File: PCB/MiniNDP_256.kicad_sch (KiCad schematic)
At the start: 18 parts, among them J1 Conn_02x20_Odd_Even, U1 74161, U2 74161, U3 74161, U4 74138, U5 74374, U6 AS6C2008A, U7 741G32

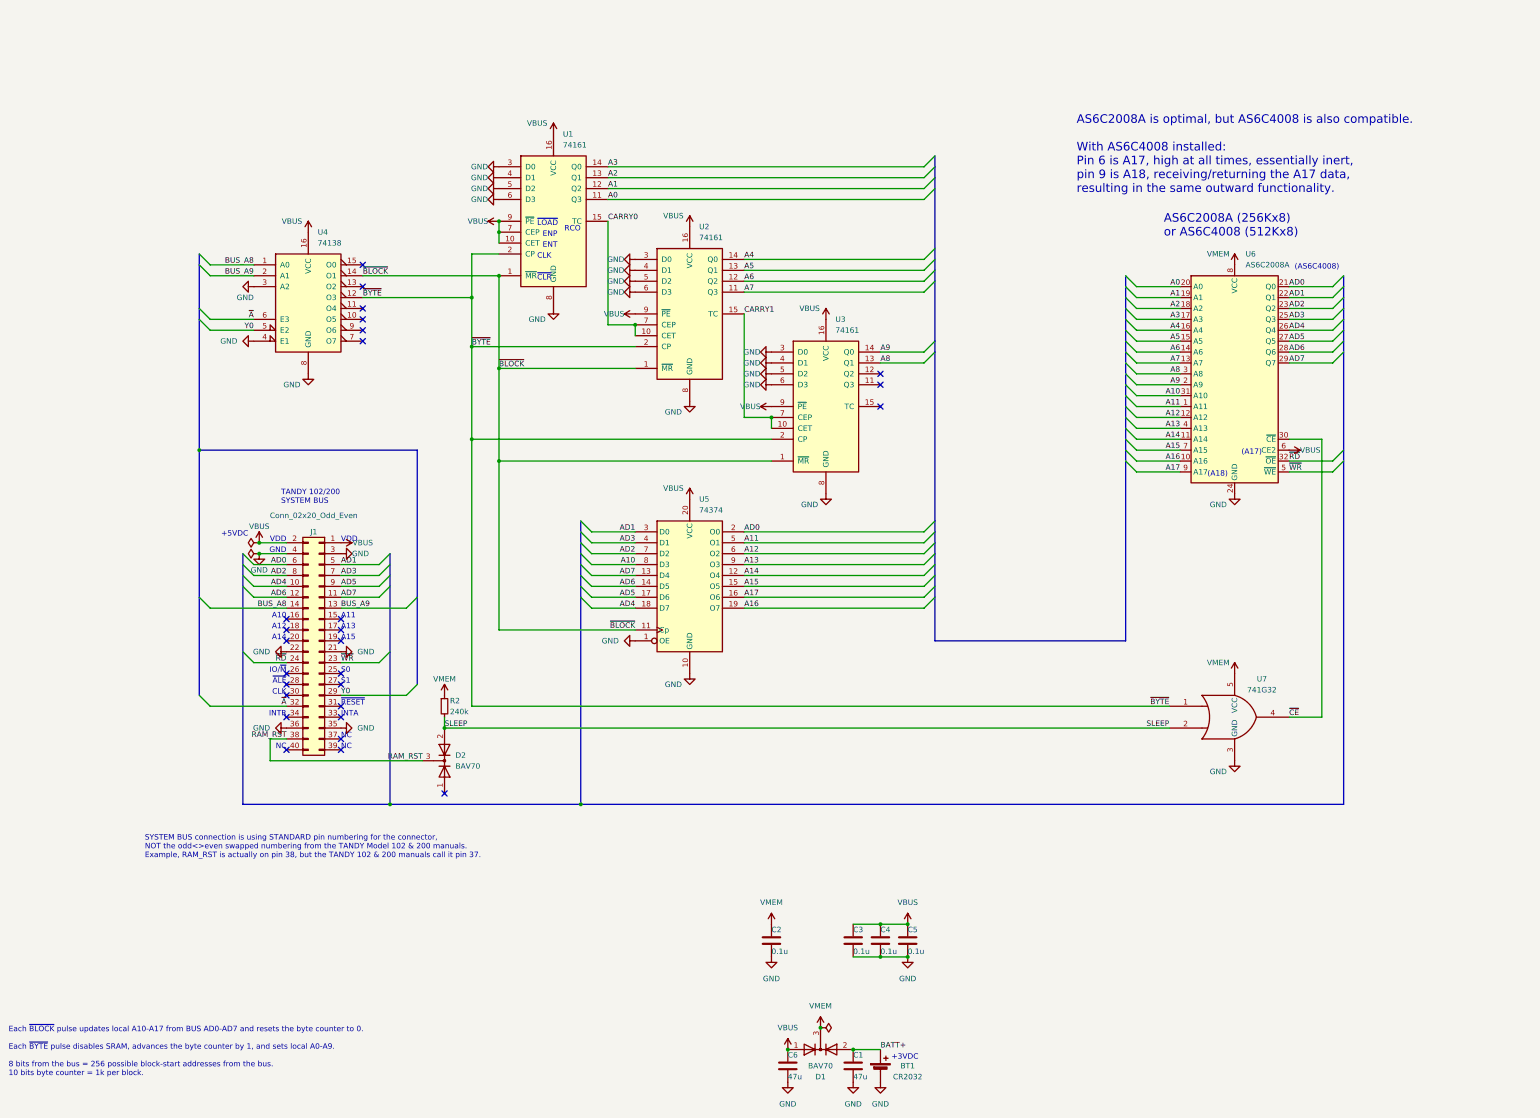
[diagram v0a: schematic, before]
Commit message: shrink MiniNDP
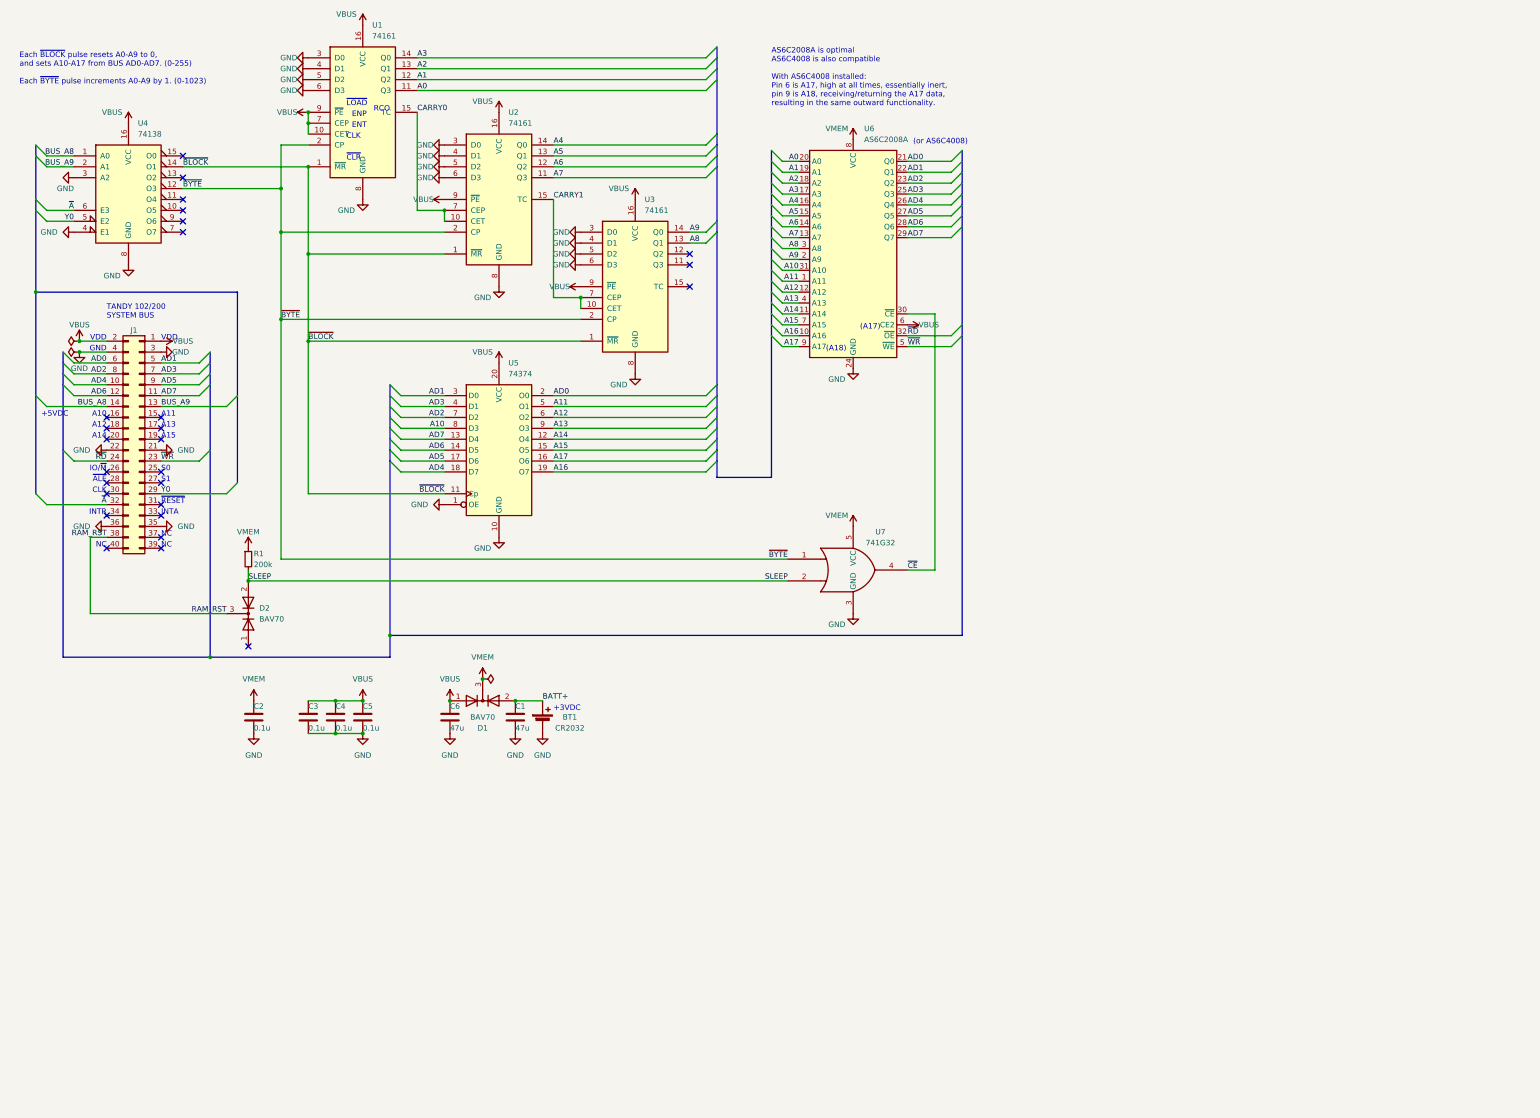
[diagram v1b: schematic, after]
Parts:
- R1: renamed from R2; value 240k -> 200k
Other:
- note added: "(or AS6C4008)"
- note added: "AS6C2008A is optimal AS6C4008 is also compatible With AS6C4008 installed: Pin 6 is A17, high at all times, essentially inert, pin 9 is A18, receiving/returning the A17 data, resulting in the same outward functionality."
- note added: "Each ~{BLOCK} pulse resets A0-A9 to 0, and sets A10-A17 from BUS AD0-AD7. (0-255) Each ~{BYTE} pulse increments A0-A9 by 1. (0-1023)"
- note removed: "(AS6C4008)"
- note removed: "AS6C2008A (256Kx8) or AS6C4008 (512Kx8)"
- note removed: "AS6C2008A is optimal, but AS6C4008 is also compatible. With AS6C4008 installed: Pin 6 is A17, high at all times, essentially inert, pin 9 is A18, receiving/returning the A17 data, resulting in the same outward functionality."
- note removed: "Each ~{BLOCK} pulse updates local A10-A17 from BUS AD0-AD7 and resets the byte counter to 0. Each ~{BYTE} pulse disables SRAM, advances the byte counter by 1, and sets local A0-A9. 8 bits from the bus = 256 possible block-start addresses from the bus. 10 bits byte counter = 1k per block."
- note removed: "SYSTEM BUS connection is using STANDARD pin numbering for the connector, NOT the odd<>even swapped numbering from the TANDY Model 102 & 200 manuals. Example, RAM_RST is actually on pin 38, but the TANDY 102 & 200 manuals call it pin 37."
- moved on the sheet: BT1, C1, C2, C3, C4, C5, C6, D1, D2, J1, R1, U1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

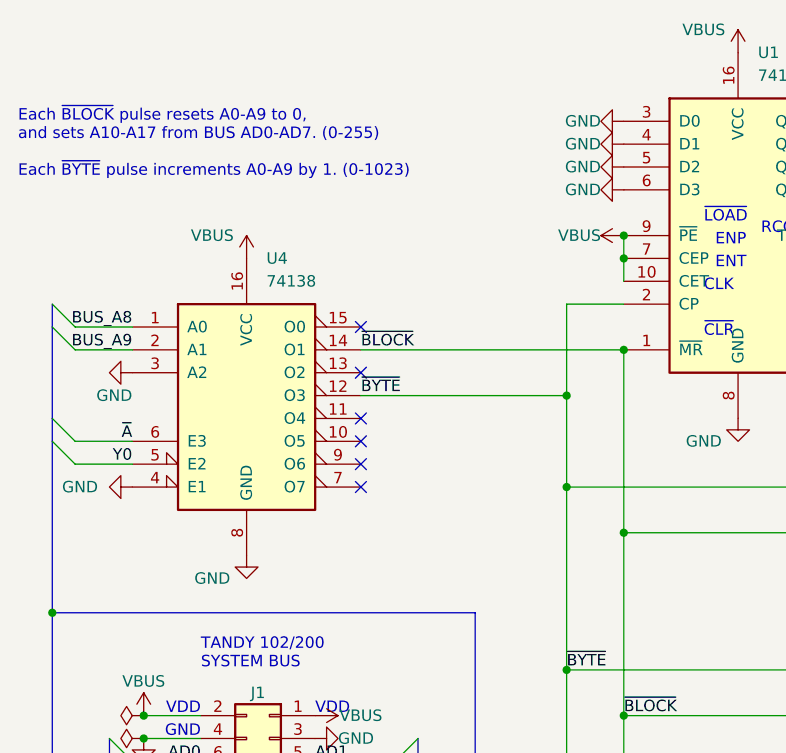
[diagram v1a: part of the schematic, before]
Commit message: minor sch alignment
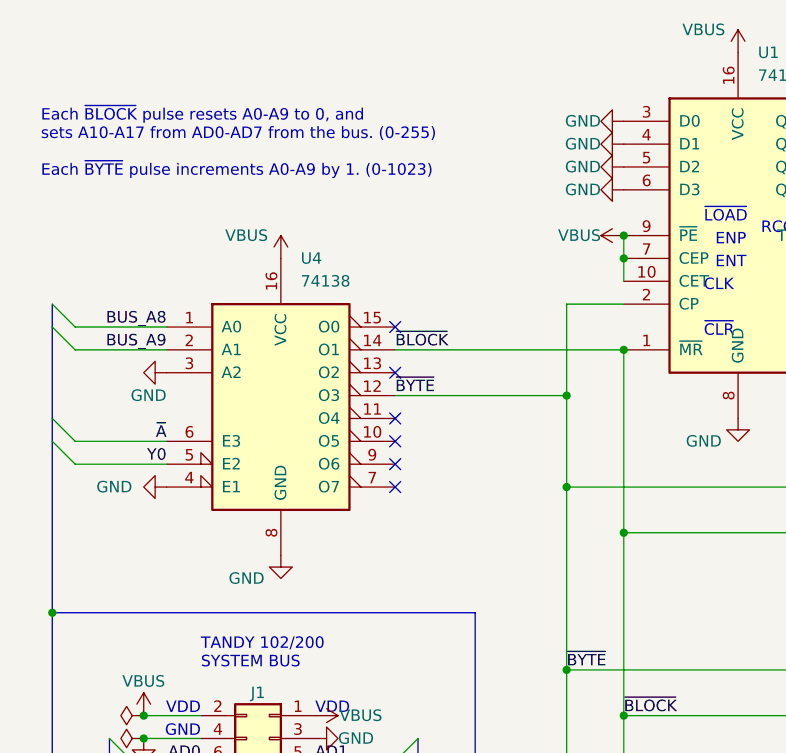
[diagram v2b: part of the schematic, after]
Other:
- note added: "Each ~{BLOCK} pulse resets A0-A9 to 0, and sets A10-A17 from AD0-AD7 from the bus. (0-255) Each ~{BYTE} pulse increments A0-A9 by 1. (0-1023)"
- note removed: "Each ~{BLOCK} pulse resets A0-A9 to 0, and sets A10-A17 from BUS AD0-AD7. (0-255) Each ~{BYTE} pulse increments A0-A9 by 1. (0-1023)"
- moved on the sheet: U4
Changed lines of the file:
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@@
   (junction (at 134.62 179.07) (diameter 0) (color 0 0 0 0)
   )
-  (no_connect (at 72.39 57.15))
+  (no_connect (at 76.2 57.15))
   (no_connect (at 67.31 133.35))
   (no_connect (at 190.5 74.93))
   (no_connect (at 67.31 118.11))
-  (no_connect (at 72.39 62.23))
+  (no_connect (at 76.2 62.23))
   (no_connect (at 54.61 143.51))
   (no_connect (at 67.31 125.73))
-  (no_connect (at 72.39 69.85))
+  (no_connect (at 76.2 69.85))
   (no_connect (at 67.31 143.51))
   (no_connect (at 190.5 77.47))
@@
   (no_connect (at 190.5 82.55))
   (no_connect (at 54.61 115.57))
-  (no_connect (at 72.39 67.31))
+  (no_connect (at 76.2 67.31))
   (no_connect (at 54.61 118.11))
   (no_connect (at 54.61 135.89))
-  (no_connect (at 72.39 64.77))
+  (no_connect (at 76.2 64.77))
   (no_connect (at 67.31 113.03))
   (no_connect (at 54.61 128.27))
@@
   (no_connect (at 87.63 166.37))
   (no_connect (at 54.61 113.03))
-  (no_connect (at 72.39 52.07))
+  (no_connect (at 76.2 52.07))
   (bus_entry (at 194.31 72.39) (size 2.54 -2.54)
     (stroke (width 0) (type default))
@@
     (stroke (width 0) (type default))
   )
-  (wire (pts (xy 40.64 67.31) (xy 46.99 67.31))
+  (wire (pts (xy 40.64 67.31) (xy 50.8 67.31))
     (stroke (width 0) (type default))
   )
@@
     (stroke (width 0) (type default))
   )
-  (wire (pts (xy 72.39 59.69) (xy 95.25 59.69))
+  (wire (pts (xy 76.2 59.69) (xy 95.25 59.69))
     (stroke (width 0) (type default))
   )
@@
     (stroke (width 0) (type default))
   )
-  (wire (pts (xy 72.39 54.61) (xy 101.6 54.61))
+  (wire (pts (xy 76.2 54.61) (xy 101.6 54.61))
     (stroke (width 0) (type default))
   )
@@
     (stroke (width 0) (type default))
   )
-  (wire (pts (xy 40.64 64.77) (xy 46.99 64.77))
+  (wire (pts (xy 40.64 64.77) (xy 50.8 64.77))
     (stroke (width 0) (type default))
   )
@@
     (stroke (width 0) (type default))
   )
-  (wire (pts (xy 40.64 52.07) (xy 46.99 52.07))
+  (wire (pts (xy 40.64 52.07) (xy 50.8 52.07))
     (stroke (width 0) (type default))
   )
@@
     (stroke (width 0) (type default))
   )
-  (wire (pts (xy 40.64 54.61) (xy 46.99 54.61))
+  (wire (pts (xy 40.64 54.61) (xy 50.8 54.61))
     (stroke (width 0) (type default))
   )
@@
     (effects (font (size 1.27 1.27)) (justify left bottom))
   )
-  (text "Each ~{BLOCK} pulse resets A0-A9 to 0,\nand sets A10-A17 from BUS AD0-AD7. (0-255)\n\nEach ~{BYTE} pulse increments A0-A9 by 1. (0-1023)\n"
-    (at 34.29 35.56 0)
+  (text "Each ~{BLOCK} pulse resets A0-A9 to 0, and\nsets A10-A17 from AD0-AD7 from the bus. (0-255)\n\nEach ~{BYTE} pulse increments A0-A9 by 1. (0-1023)\n"
+    (at 36.83 35.56 0)
     (effects (font (size 1.27 1.27)) (justify left bottom))
   )
@@
     (effects (font (size 1.27 1.27)) (justify right bottom))
   )
-  (label "Y0" (at 46.99 67.31 180) (fields_autoplaced)
+  (label "Y0" (at 50.8 67.31 180) (fields_autoplaced)
     (effects (font (size 1.27 1.27)) (justify right bottom))
   )
@@
     (effects (font (size 1.27 1.27)) (justify left bottom))
   )
-  (label "~{BLOCK}" (at 72.39 54.61 0) (fields_autoplaced)
+  (label "~{BLOCK}" (at 76.2 54.61 0) (fields_autoplaced)
     (effects (font (size 1.27 1.27)) (justify left bottom))
   )
@@
     (effects (font (size 1.27 1.27)) (justify right bottom))
   )
-  (label "~{A}" (at 46.99 64.77 180) (fields_autoplaced)
+  (label "~{A}" (at 50.8 64.77 180) (fields_autoplaced)
     (effects (font (size 1.27 1.27)) (justify right bottom))
   )
@@
     (effects (font (size 1.27 1.27)) (justify left bottom))
   )
-  (label "BUS_A9" (at 46.99 54.61 180) (fields_autoplaced)
+  (label "BUS_A9" (at 50.8 54.61 180) (fields_autoplaced)
     (effects (font (size 1.27 1.27)) (justify right bottom))
   )
@@
     (effects (font (size 1.27 1.27)) (justify right bottom))
   )
-  (label "BUS_A8" (at 46.99 52.07 180) (fields_autoplaced)
+  (label "BUS_A8" (at 50.8 52.07 180) (fields_autoplaced)
     (effects (font (size 1.27 1.27)) (justify right bottom))
   )
@@
     (effects (font (size 1.27 1.27)) (justify left bottom))
   )
-  (label "~{BYTE}" (at 72.39 59.69 0) (fields_autoplaced)
+  (label "~{BYTE}" (at 76.2 59.69 0) (fields_autoplaced)
     (effects (font (size 1.27 1.27)) (justify left bottom))
   )
@@
     )
   )
-  (symbol (lib_id "power:GND") (at 59.69 77.47 0) (unit 1)
-    (in_bom yes) (on_board yes) (dnp no)
-    (property "Reference" "#PWR022" (at 59.69 83.82 0)
-      (effects (font (size 1.27 1.27)) hide)
-    )
-    (property "Value" "GND" (at 55.88 80.01 0)
-      (effects (font (size 1.27 1.27)))
-    )
-    (property "Footprint" "" (at 59.69 77.47 0)
-      (effects (font (size 1.27 1.27)) hide)
-    )
-    (property "Datasheet" "" (at 59.69 77.47 0)
+  (symbol (lib_id "power:GND") (at 63.5 77.47 0) (unit 1)
+    (in_bom yes) (on_board yes) (dnp no)
+    (property "Reference" "#PWR022" (at 63.5 83.82 0)
+      (effects (font (size 1.27 1.27)) hide)
+    )
+    (property "Value" "GND" (at 59.69 80.01 0)
+      (effects (font (size 1.27 1.27)))
+    )
+    (property "Footprint" "" (at 63.5 77.47 0)
+      (effects (font (size 1.27 1.27)) hide)
+    )
+    (property "Datasheet" "" (at 63.5 77.47 0)
       (effects (font (size 1.27 1.27)) hide)
     )
@@
     )
   )
-  (symbol (lib_id "power:GND") (at 46.99 57.15 270) (unit 1)
-    (in_bom yes) (on_board yes) (dnp no)
-    (property "Reference" "#PWR037" (at 40.64 57.15 0)
-      (effects (font (size 1.27 1.27)) hide)
-    )
-    (property "Value" "GND" (at 46.99 59.69 90)
+  (symbol (lib_id "power:GND") (at 50.8 57.15 270) (unit 1)
+    (in_bom yes) (on_board yes) (dnp no)
+    (property "Reference" "#PWR037" (at 44.45 57.15 0)
+      (effects (font (size 1.27 1.27)) hide)
+    )
+    (property "Value" "GND" (at 50.8 59.69 90)
       (effects (font (size 1.27 1.27)) (justify right))
     )
-    (property "Footprint" "" (at 46.99 57.15 0)
-      (effects (font (size 1.27 1.27)) hide)
-    )
-    (property "Datasheet" "" (at 46.99 57.15 0)
+    (property "Footprint" "" (at 50.8 57.15 0)
+      (effects (font (size 1.27 1.27)) hide)
+    )
+    (property "Datasheet" "" (at 50.8 57.15 0)
       (effects (font (size 1.27 1.27)) hide)
     )
@@
     )
   )
-  (symbol (lib_id "000_LOCAL:74138") (at 59.69 59.69 0) (unit 1)
+  (symbol (lib_id "000_LOCAL:74138") (at 63.5 59.69 0) (unit 1)
     (in_bom yes) (on_board yes) (dnp no) (fields_autoplaced)
-    (property "Reference" "U4" (at 61.8841 44.45 0)
+    (property "Reference" "U4" (at 65.6941 44.45 0)
       (effects (font (size 1.27 1.27)) (justify left))
     )
-    (property "Value" "74138" (at 61.8841 46.99 0)
+    (property "Value" "74138" (at 65.6941 46.99 0)
       (effects (font (size 1.27 1.27)) (justify left))
     )
-    (property "Footprint" "000_LOCAL:TSSOP-16" (at 59.69 59.69 0)
-      (effects (font (size 1.27 1.27)) hide)
-    )
-    (property "Datasheet" "datasheets/74HC138.pdf" (at 59.69 59.69 0)
+    (property "Footprint" "000_LOCAL:TSSOP-16" (at 63.5 59.69 0)
+      (effects (font (size 1.27 1.27)) hide)
+    )
+    (property "Datasheet" "datasheets/74HC138.pdf" (at 63.5 59.69 0)
       (effects (font (size 1.27 1.27)) hide)
     )
@@
     )
   )
-  (symbol (lib_id "power:GND") (at 46.99 69.85 270) (unit 1)
+  (symbol (lib_id "power:GND") (at 50.8 69.85 270) (unit 1)
     (in_bom yes) (on_board yes) (dnp no) (fields_autoplaced)
-    (property "Reference" "#PWR038" (at 40.64 69.85 0)
-      (effects (font (size 1.27 1.27)) hide)
-    )
-    (property "Value" "GND" (at 43.18 69.85 90)
+    (property "Reference" "#PWR038" (at 44.45 69.85 0)
+      (effects (font (size 1.27 1.27)) hide)
+    )
+    (property "Value" "GND" (at 46.99 69.85 90)
       (effects (font (size 1.27 1.27)) (justify right))
     )
-    (property "Footprint" "" (at 46.99 69.85 0)
-      (effects (font (size 1.27 1.27)) hide)
-    )
-    (property "Datasheet" "" (at 46.99 69.85 0)
+    (property "Footprint" "" (at 50.8 69.85 0)
+      (effects (font (size 1.27 1.27)) hide)
+    )
+    (property "Datasheet" "" (at 50.8 69.85 0)
       (effects (font (size 1.27 1.27)) hide)
     )
@@
     )
   )
-  (symbol (lib_id "power:VBUS") (at 59.69 44.45 0) (unit 1)
-    (in_bom yes) (on_board yes) (dnp no)
-    (property "Reference" "#PWR033" (at 59.69 48.26 0)
-      (effects (font (size 1.27 1.27)) hide)
-    )
-    (property "Value" "VBUS" (at 55.88 41.91 0)
-      (effects (font (size 1.27 1.27)))
-    )
-    (property "Footprint" "" (at 59.69 44.45 0)
-      (effects (font (size 1.27 1.27)) hide)
-    )
-    (property "Datasheet" "" (at 59.69 44.45 0)
-      (effects (font (size 1.27 1.27)) hide)
-    )
+  (symbol (lib_id "power:VBUS") (at 63.5 44.45 0) (unit 1)
+    (in_bom yes) (on_board yes) (dnp no)
+    (property "Reference" "#PWR033" (at 63.5 48.26 0)
+      (effects (font (size 1.27 1.27)) hide)
+    )
+    (property "Value" "VBUS" (at 59.69 41.91 0)
+      (effects (font (size 1.27 1.27)))
+    )
+    (property "Footprint" "" (at 63.5 44.45 0)
+      (effects (font (size 1.27 1.27)) hide)
+    )
+    (property "Datasheet" "" (at 63.5 44.45 0)
+      (effects (font (size 1.27 1.27)) hide)
+    )
